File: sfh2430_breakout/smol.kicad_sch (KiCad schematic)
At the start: 3 parts, among them J6 Conn_01x01, J7 Conn_01x01

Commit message: ordered sfh2430 breakout rev 0.1
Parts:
- D1: footprint OptoDevice:Osram_SFH2430 -> adcs:Osram_SFH2430
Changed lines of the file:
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@@
       (effects (font (size 1.27 1.27)) (justify left))
     )
-    (property "Footprint" "OptoDevice:Osram_SFH2430" (at 158.1404 89.3572 0)
+    (property "Footprint" "adcs:Osram_SFH2430" (at 158.1404 89.3572 0)
       (effects (font (size 1.27 1.27)) hide)
     )
@@
       (effects (font (size 1.27 1.27)) hide)
     )
+    (property "DigiKey Part Number" "" (at 153.6954 89.3572 0)
+      (effects (font (size 1.27 1.27)) hide)
+    )
+    (property "Tolerance" "" (at 153.6954 89.3572 0)
+      (effects (font (size 1.27 1.27)))
+    )
+    (property "Power Rating" "" (at 153.6954 89.3572 0)
+      (effects (font (size 1.27 1.27)))
+    )
     (pin "1")

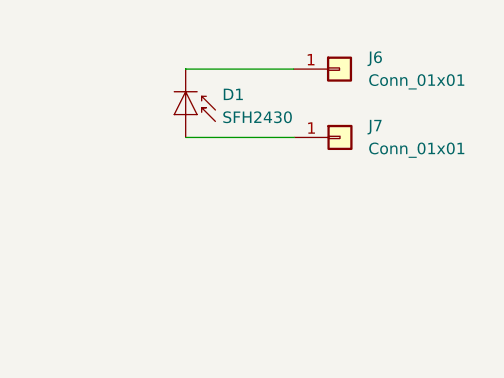
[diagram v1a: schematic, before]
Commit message: sfh2400 v2 (flex PCB)
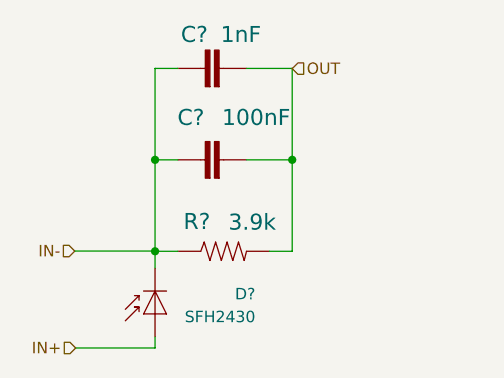
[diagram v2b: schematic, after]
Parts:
- removed D1: SFH2430, adcs:Osram_SFH2430, symbol Sensor_Optical:SFH2430
- removed J6, J7: Conn_01x01, adcs:castellated_05mm, symbol Connector_Generic:Conn_01x01
- added C?: 100nF, Capacitor_SMD:C_0603_1608Metric, symbol mainboard:22UF-1210-16V-20%
- added C?: 1nF, Capacitor_SMD:C_0603_1608Metric, symbol mainboard:22UF-1210-16V-20%
- added D?: SFH2430, adcs:Osram_SFH2430, symbol Sensor_Optical:SFH2430
- added R?: 3.9k, Resistor_SMD:R_0603_1608Metric, symbol pycubed_mainboard:RESISTOR0603
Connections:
- new net IN+: D?.2 (A)
- new net IN-: C?.1, C?.1, D?.1 (K), R?.1
- new net OUT: C?.2, C?.2, R?.2
